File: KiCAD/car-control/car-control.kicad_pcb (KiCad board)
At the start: 2 copper layers, 171.4 x 40 mm, 23 parts, among them J1 USB_B_Micro, J2 Conn_01x06, J3 USB_A, J4 Conn_01x04, SW1 SW_Push, SW2 SW_Push, SW3 SW_Push, SW4 SW_Push, SW5 COM-15140, U1 OLED-SSD1322

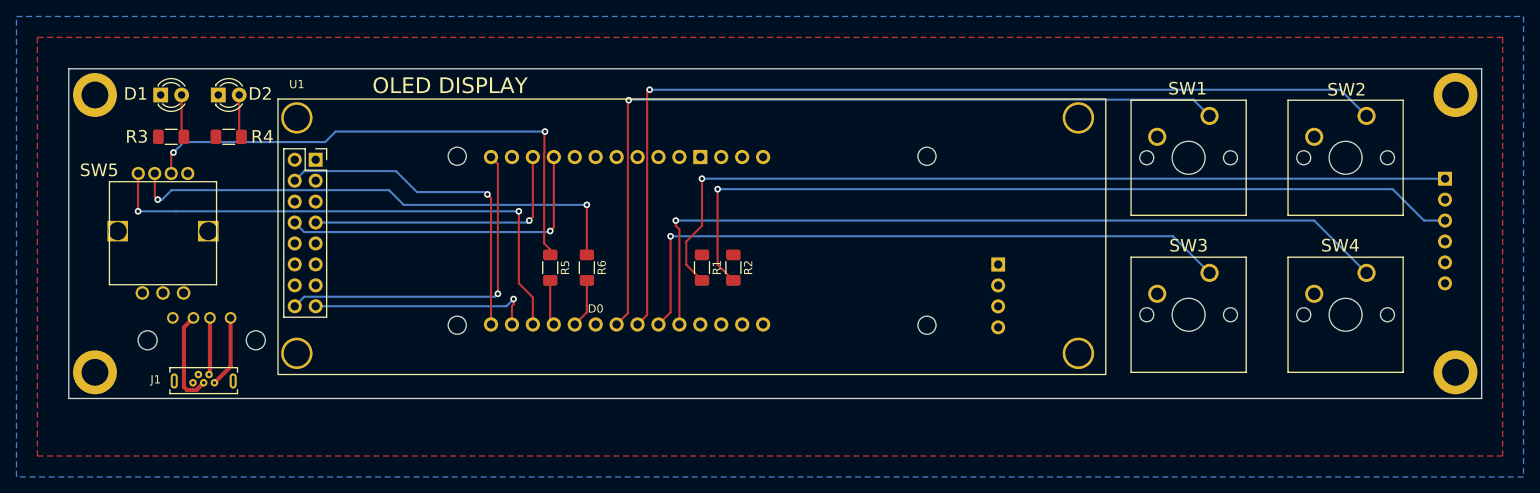
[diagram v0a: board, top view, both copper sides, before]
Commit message: working on layout, move USB
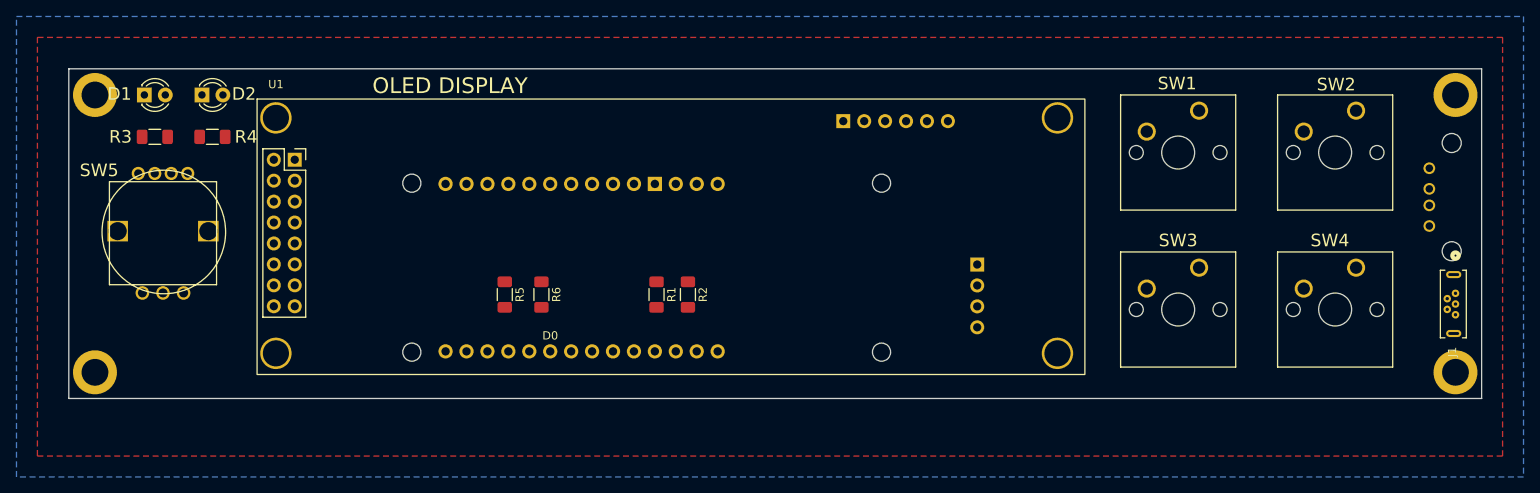
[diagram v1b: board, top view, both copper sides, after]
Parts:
- moved J1 151.0 mm to (243.2, 76.8), turned to -90 degrees
- moved J3 146.6 mm to (240.0, 61.6), turned to -90 degrees
- moved J2 73.4 mm to (168.9, 55.9), turned to -90 degrees
- moved R1 6.41 mm to (146.2, 76.9)
- moved R2 6.41 mm to (150.1, 76.9)
- moved R5 6.41 mm to (127.8, 76.9)
- moved R6 6.41 mm to (132.3, 76.9)
- moved A1 6.41 mm to (173.6, 63.4)
- moved U1 2.54 mm to (97.8, 53.2)
- moved J4 2.54 mm to (185.2, 73.3)
- moved D1 1.98 mm to (84.1, 52.7)
- moved D2 1.98 mm to (91.1, 52.7)
- moved R3 1.98 mm to (85.4, 57.8)
- moved R4 1.98 mm to (92.4, 57.8)
- moved SW3 1.42 mm to (212.1, 73.7)
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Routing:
- net /SW1: track 117.4 -> 0.00 mm, vias 1 -> 0
- net /A0: track 104.1 -> 0.00 mm, vias 1 -> 0
- net /A1: track 101.7 -> 0.00 mm, vias 1 -> 0
- net /SW3: track 99.2 -> 0.00 mm, vias 1 -> 0
- net /SW0: track 99.2 -> 0.00 mm, vias 1 -> 0
- net /SW2: track 78.6 -> 0.00 mm, vias 1 -> 0
- net /ENC_SW: track 65.5 -> 0.00 mm, vias 2 -> 0
- net Net-(SW5-RED): track 64.1 -> 0.00 mm, vias 2 -> 0
- net Net-(SW5-GREEN): track 62.7 -> 0.00 mm, vias 2 -> 0
- net /~{RST}: track 42.2 -> 0.00 mm, vias 1 -> 0
- net /DC: track 41.0 -> 0.00 mm, vias 1 -> 0
- net /SCK: track 40.7 -> 0.00 mm, vias 1 -> 0
- net /MOSI: track 33.9 -> 0.00 mm, vias 1 -> 0
- net /~{CS}: track 27.5 -> 0.00 mm, vias 1 -> 0
- net Net-(J1-D+): track 11.8 -> 0.00 mm
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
